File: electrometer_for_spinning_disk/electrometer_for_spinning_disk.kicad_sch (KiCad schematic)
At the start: 25 parts, among them J2 Conn_01x03_Pin, J3 Screw_Terminal_01x03, J4 PRT-14417, J6 Conn_01x03_Pin, J7 Conn_01x03_Pin, U1 LMC6082, U2 ADS1115IDGS, U3 REF3025, U4 5V LDO, U5 INA159AIDGKR

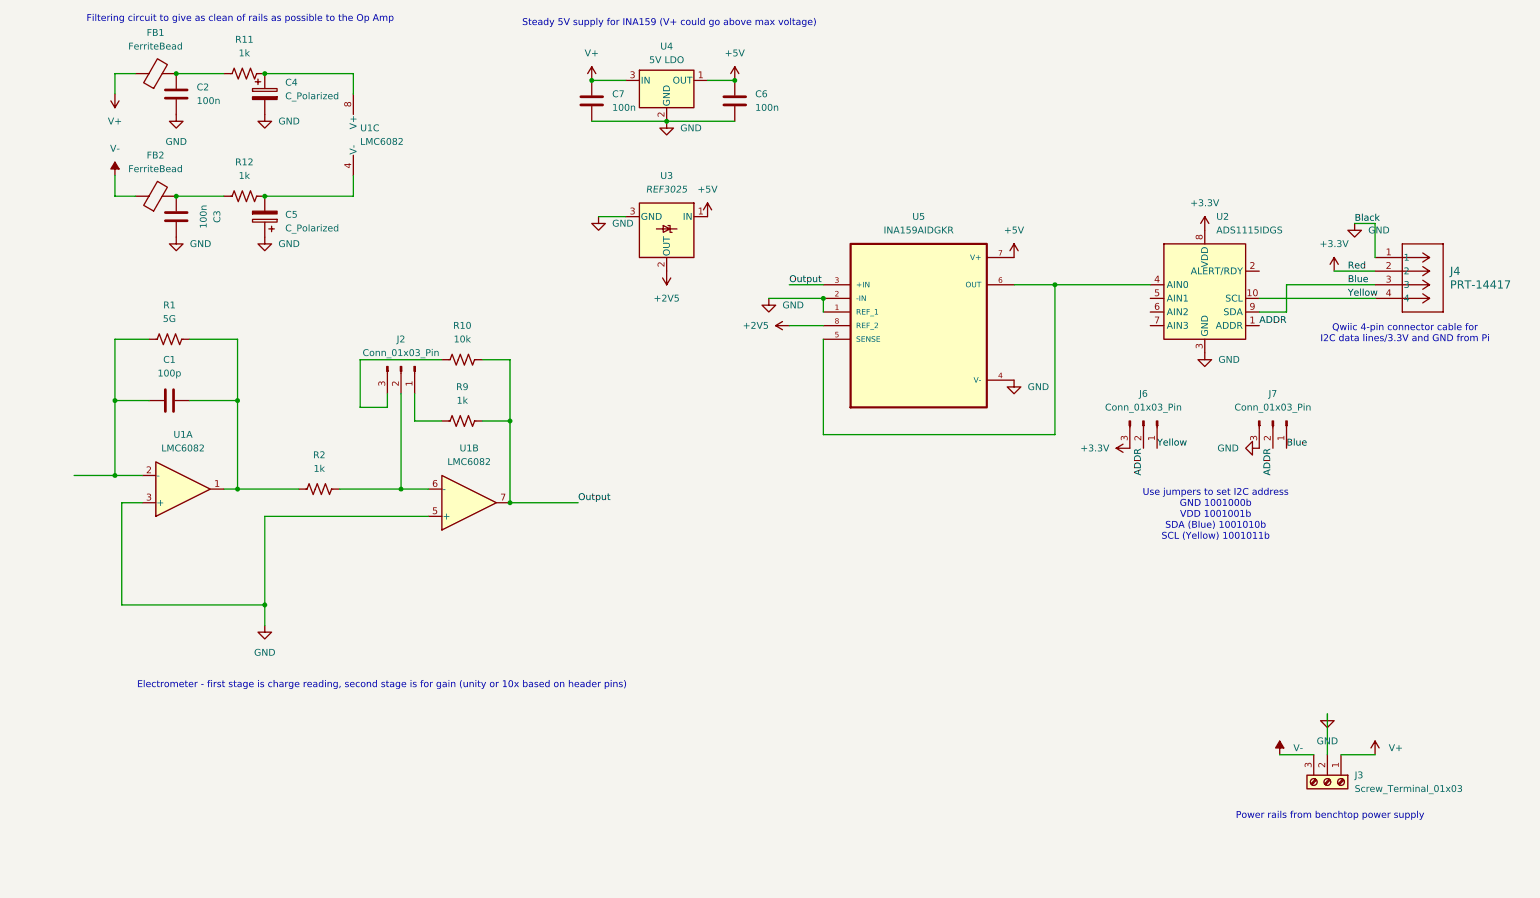
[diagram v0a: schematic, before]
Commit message: so much! I should push more!
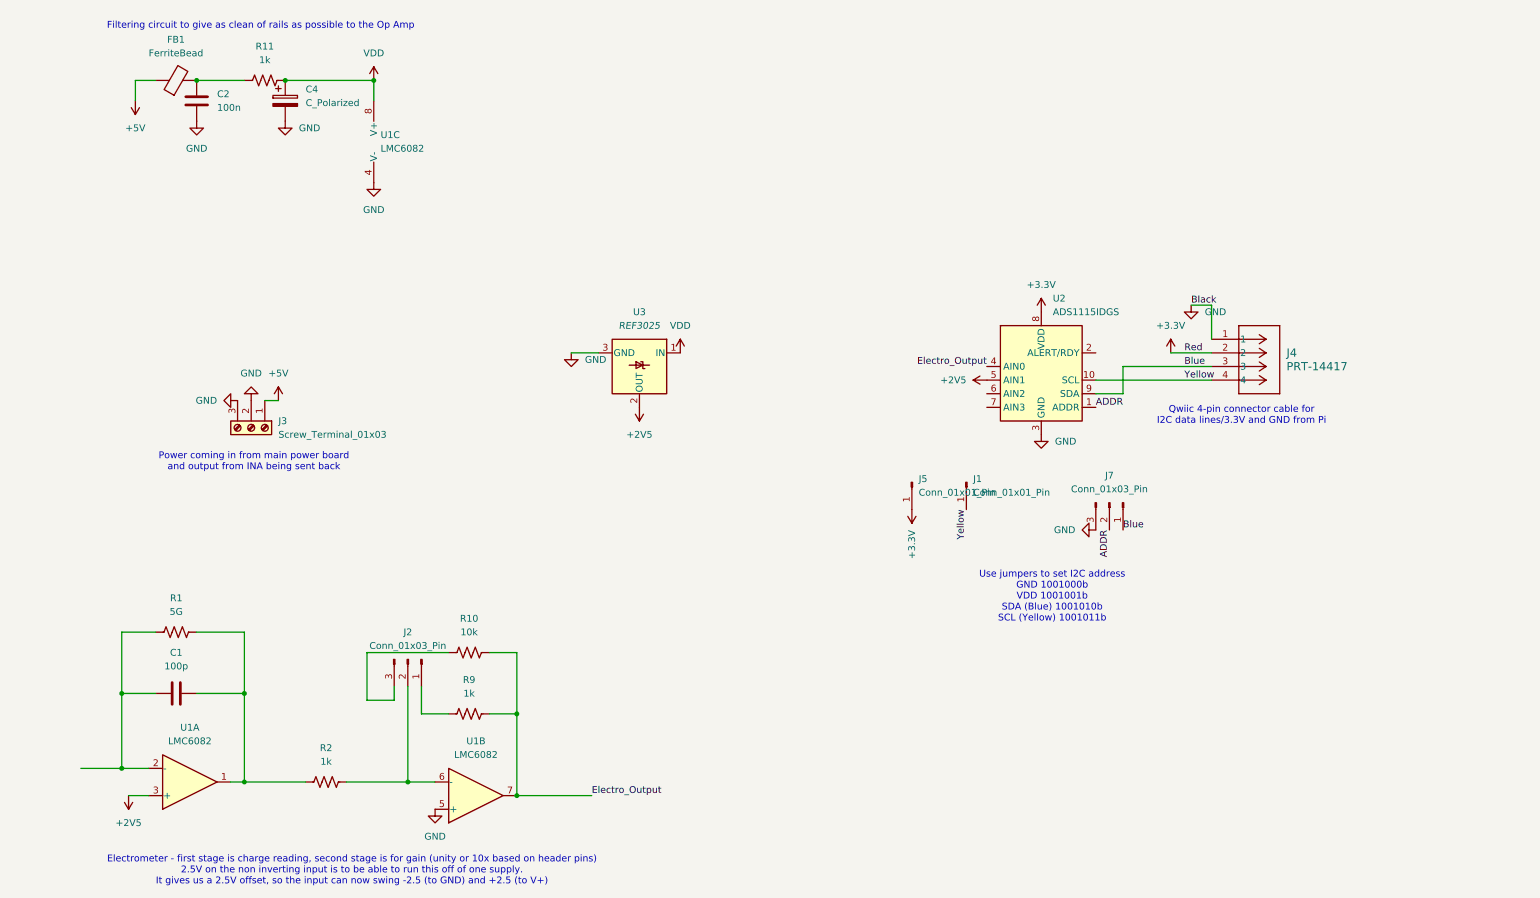
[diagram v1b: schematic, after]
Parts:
- removed C3, C6, C7: 100n, Capacitor_SMD:C_1206_3216Metric, symbol Device:C
- removed C5: C_Polarized, Capacitor_SMD:CP_Elec_10x10.5, symbol Device:C_Polarized
- removed FB2: FerriteBead, Inductor_SMD:L_1206_3216Metric, symbol Device:FerriteBead
- removed J6: Conn_01x03_Pin, Connector_PinHeader_2.54mm:PinHeader_1x03_P2.54mm_Vertical, symbol Connector:Conn_01x03_Pin
- removed R12: 1k, Resistor_SMD:R_1206_3216Metric_Pad1.30x1.75mm_HandSolder, symbol Device:R_US
- removed U4: 5V LDO, Package_TO_SOT_SMD:SOT-89-3, symbol Regulator_Linear:L78L08_SOT89
- removed U5: INA159AIDGKR, Package_SO:TSSOP-8_3x3mm_P0.65mm, symbol ADS8681:INA159AIDGKR
- added J1, J5: Conn_01x01_Pin, Connector_PinHeader_2.54mm:PinHeader_1x01_P2.54mm_Vertical, symbol Connector:Conn_01x01_Pin
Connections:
- net Output is gone; now on net Electro_Output: R10.2, R9.2, U1.7
- net V+ is gone; now on net +5V: FB1.1, J3.1 (Pin_1)
- net V- is gone; now on net GND: J3.3 (Pin_3)
- net +2V5: now also U1.3 (+), U2.5 (AIN1)
- net +3.3V: now also J5.1 (Pin_1)
- net +5V: no longer U3.1 (IN)
- net GND: now also U1.4 (V-); no longer U1.3 (+)
- net Yellow: now also J1.1 (Pin_1)
- net Electro_Output: now reaches U2.4 (AIN0)
- net VDD: now reaches C4.1, R11.2, U1.8 (V+)
- net VDD: now also U3.1 (IN)
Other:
- note added: "Electrometer - first stage is charge reading, second stage is for gain (unity or 10x based on header pins) 2.5V on the non inverting input is to be able to run this off of one supply. It gives us a 2.5V offset, so the input can now swing -2.5 (to GND) and +2.5 (to V+)"
- note added: "Power coming in from main power board and output from INA being sent back"
- note removed: "Electrometer - first stage is charge reading, second stage is for gain (unity or 10x based on header pins)"
- note removed: "Power rails from benchtop power supply"
- note removed: "Steady 5V supply for INA159 (V+ could go above max voltage)"
